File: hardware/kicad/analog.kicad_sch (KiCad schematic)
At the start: 9 parts, among them U5 MAX4238ASA

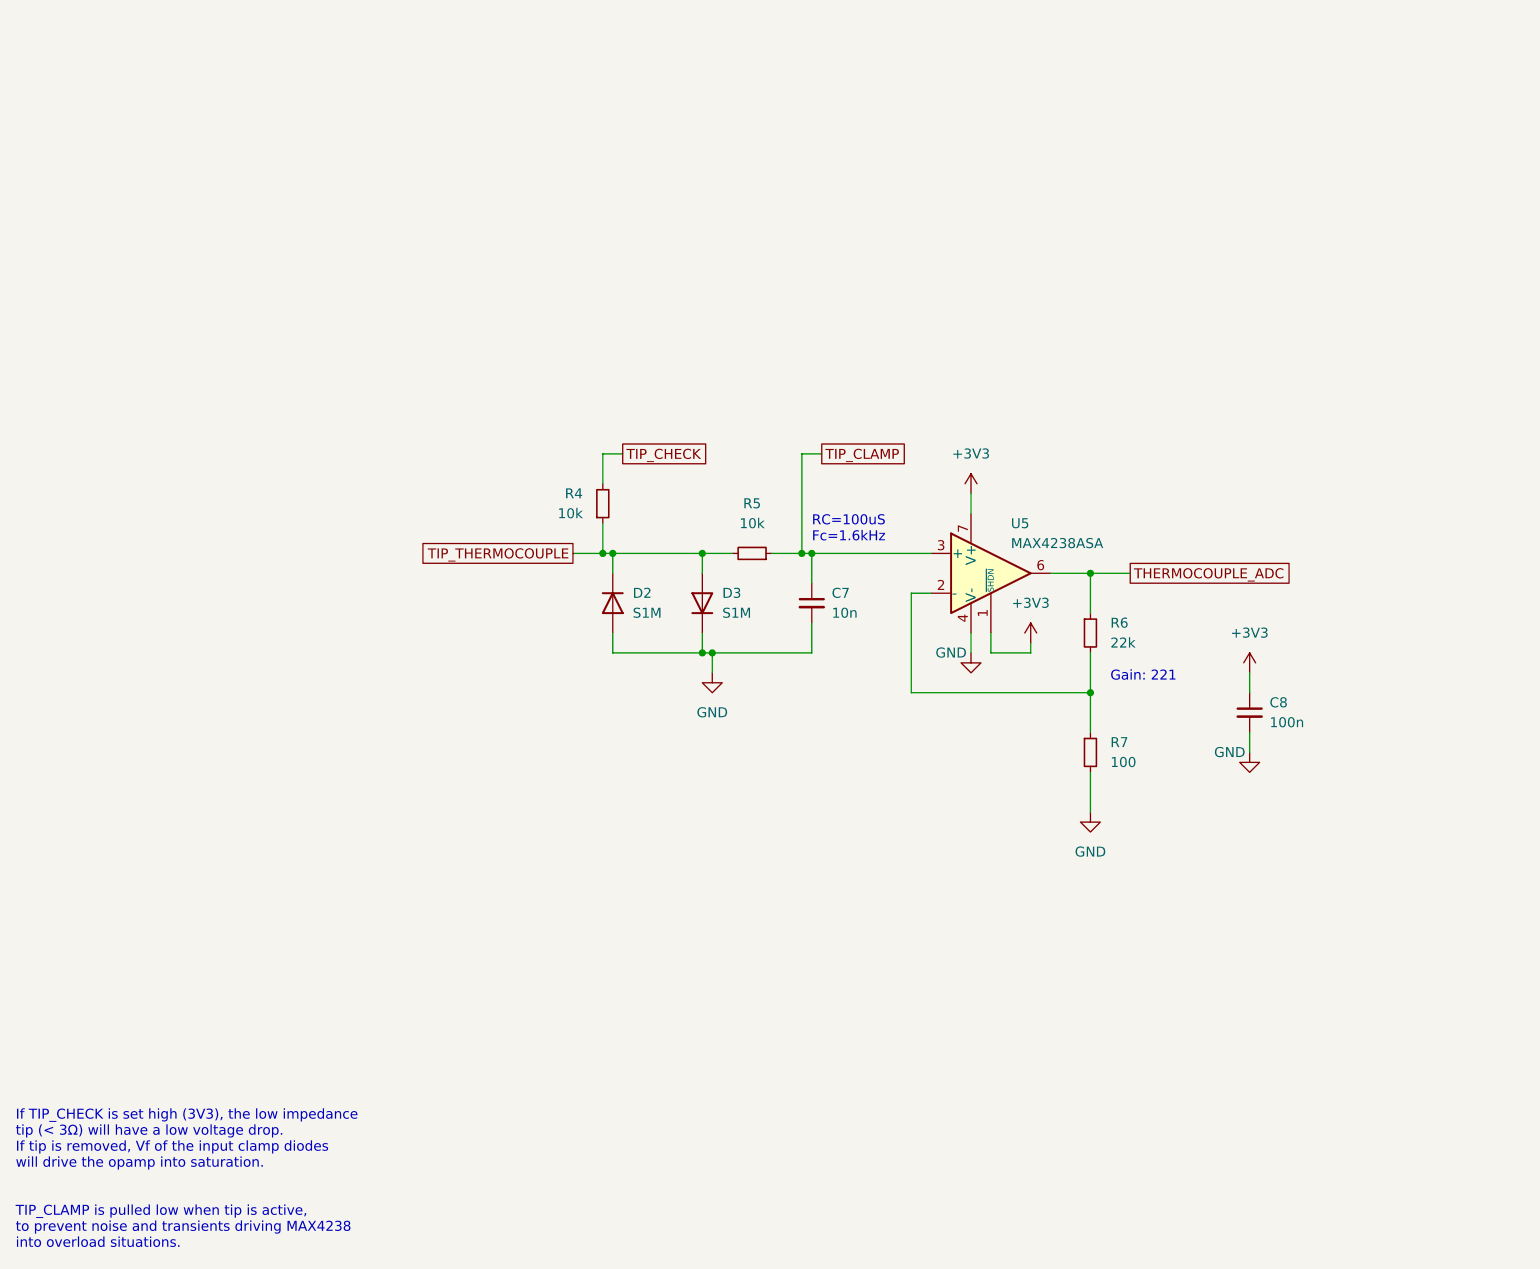
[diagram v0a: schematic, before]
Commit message: Schematic update.
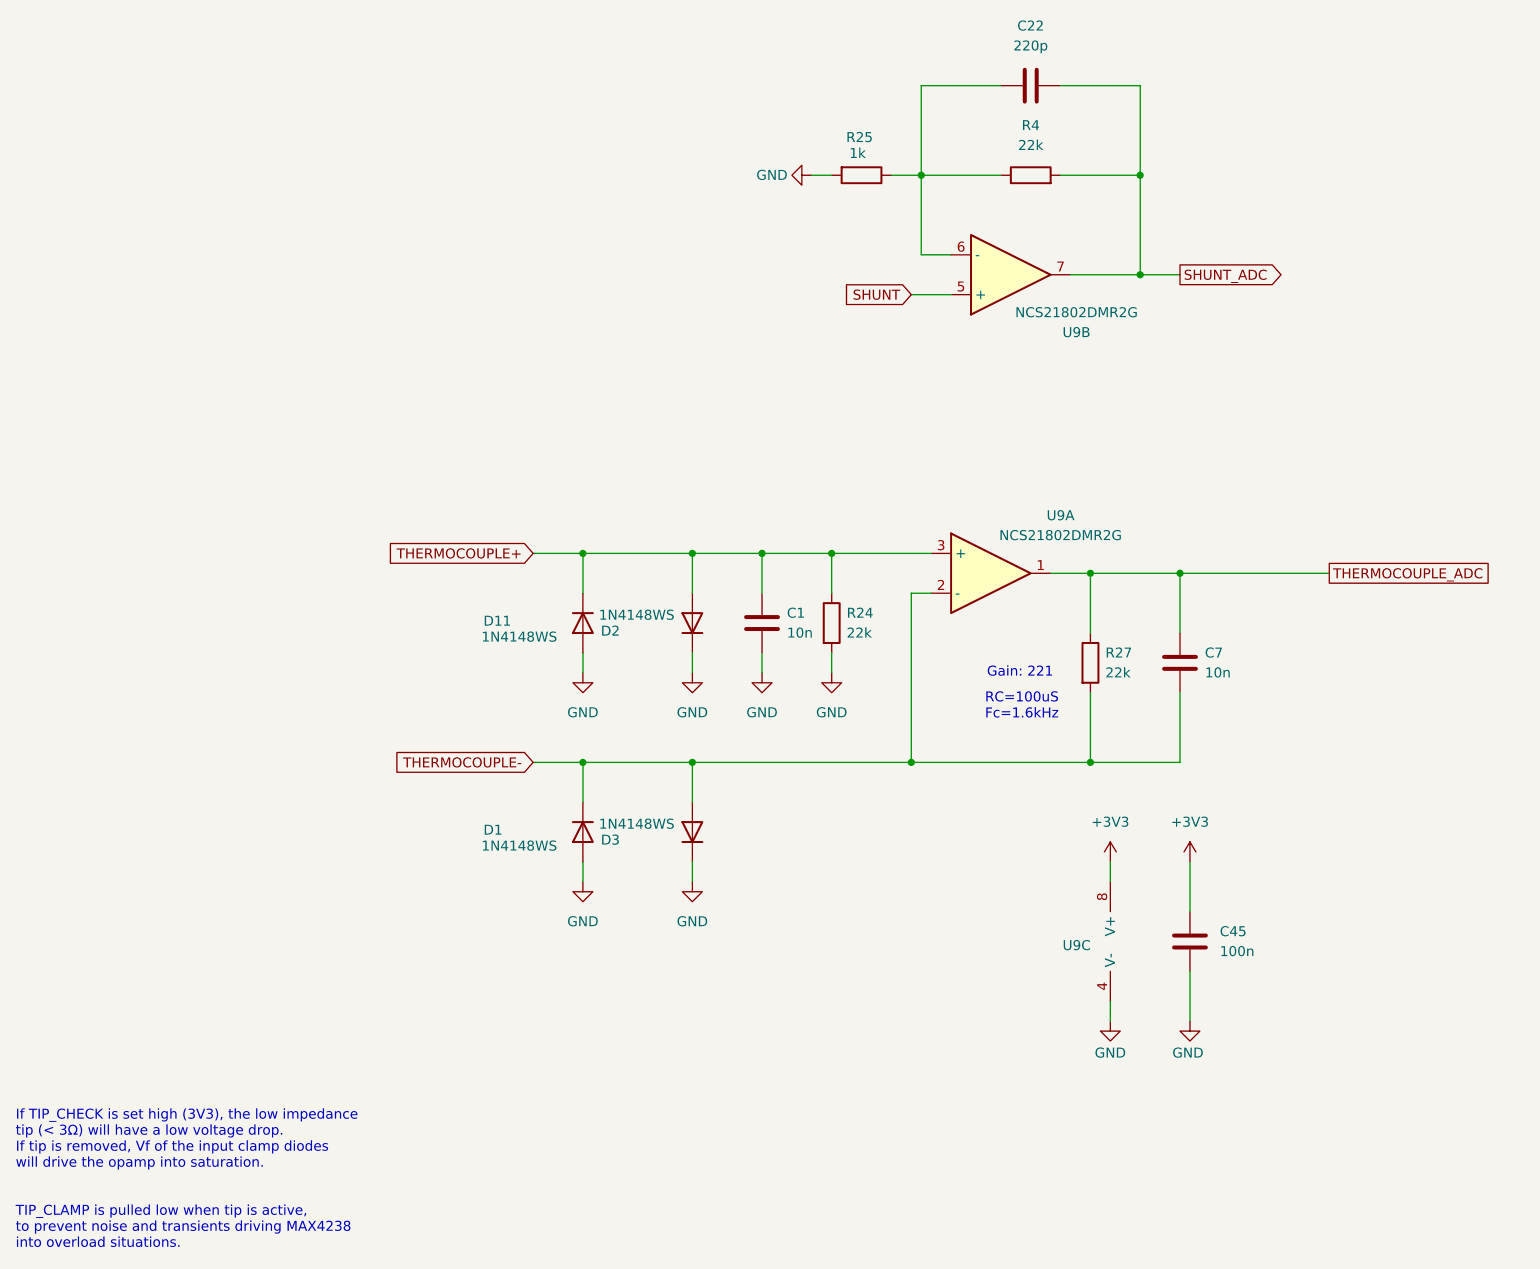
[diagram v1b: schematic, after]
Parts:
- removed C7: 10n, Capacitor_SMD:C_0805_2012Metric, symbol Device:C_Small
- removed C8: 100n, Capacitor_SMD:C_0805_2012Metric, symbol Device:C_Small
- removed D2, D3: S1M, Diode_SMD:D_SMA, symbol 0_Howie:S1M
- removed R4, R5: 10k, Resistor_SMD:R_0805_2012Metric, symbol Device:R_Small
- removed R6: 22k, Resistor_SMD:R_0805_2012Metric, symbol Device:R_Small
- removed R7: 100, Resistor_SMD:R_0805_2012Metric, symbol Device:R_Small
- removed U5: MAX4238ASA, Package_SO:SOIC-8_3.9x4.9mm_P1.27mm, symbol Amplifier_Operational:MAX4238ASA
- added C1, C7: 10n, Capacitor_SMD:C_0603_1608Metric_Pad1.08x0.95mm_HandSolder, symbol Device:C
- added C22: 220p, Capacitor_SMD:C_0603_1608Metric_Pad1.08x0.95mm_HandSolder, symbol Device:C
- added C45: 100n, Capacitor_SMD:C_0603_1608Metric_Pad1.08x0.95mm_HandSolder, symbol Device:C
- added D1, D11, D2, D3: 1N4148WS, Diode_SMD:D_SOD-323, symbol Diode:1N4148WS
- added R24, R27, R4: 22k, Resistor_SMD:R_0603_1608Metric_Pad0.98x0.95mm_HandSolder, symbol Device:R
- added R25: 1k, Resistor_SMD:R_0603_1608Metric_Pad0.98x0.95mm_HandSolder, symbol Device:R
- added U9: NCS21802DMR2G, Package_SO:OnSemi_Micro8, symbol voltmeter_lib:NCS21802DMR2G
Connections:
- net +3V3: now also C45.2, U9.8 (V+)
- net GND: now also C1.1, C45.1, D1.2 (A), D11.2 (A), D2.1 (K), D3.1 (K), R24.2, R25.2, U9.4 (V-)
- net THERMOCOUPLE_ADC: now also C7.2, R27.1, U9.1
- new net: C22.1, R25.1, R4.1, U9.6 (-)
- new net SHUNT: U9.5 (+)
- new net SHUNT_ADC: C22.2, R4.2, U9.7
- new net THERMOCOUPLE+: C1.2, D11.1 (K), D2.2 (A), R24.1, U9.3 (+)
- new net THERMOCOUPLE-: C7.1, D1.1 (K), D3.2 (A), R27.2, U9.2 (-)
